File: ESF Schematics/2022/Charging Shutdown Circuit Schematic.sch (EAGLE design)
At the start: 15 parts, among them K1 RELAY_SPST_NO_

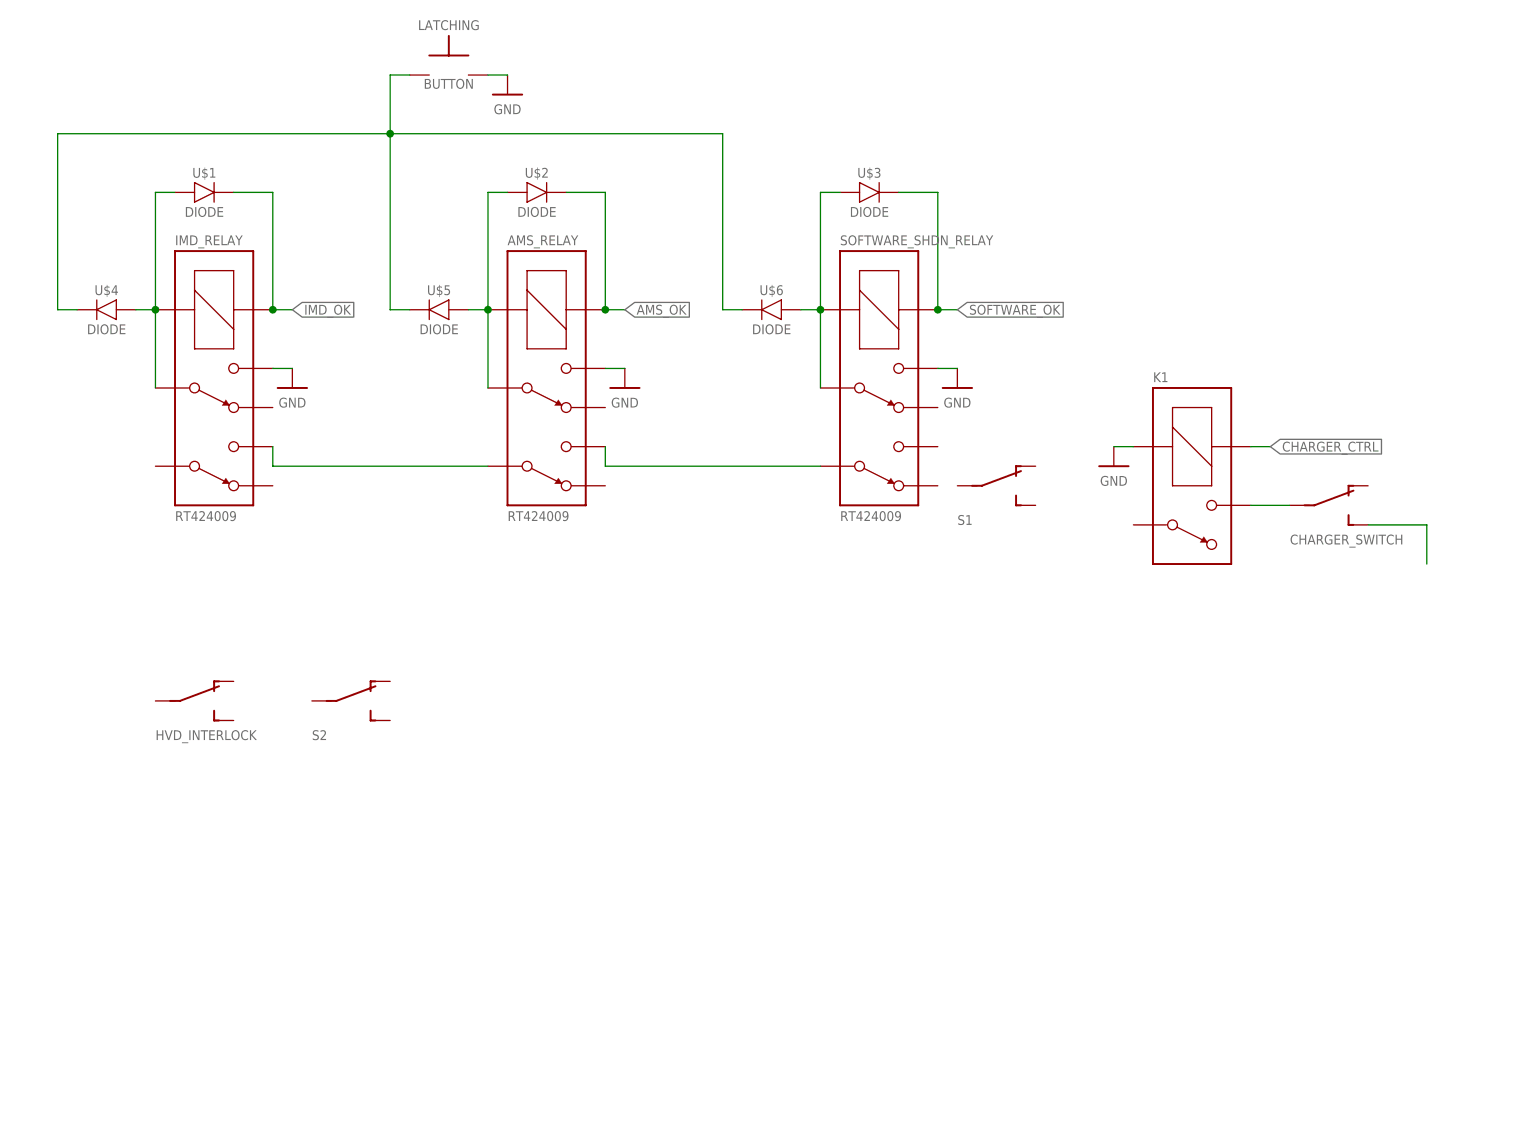
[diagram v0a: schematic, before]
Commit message: Further progress on charging shutdown circuit
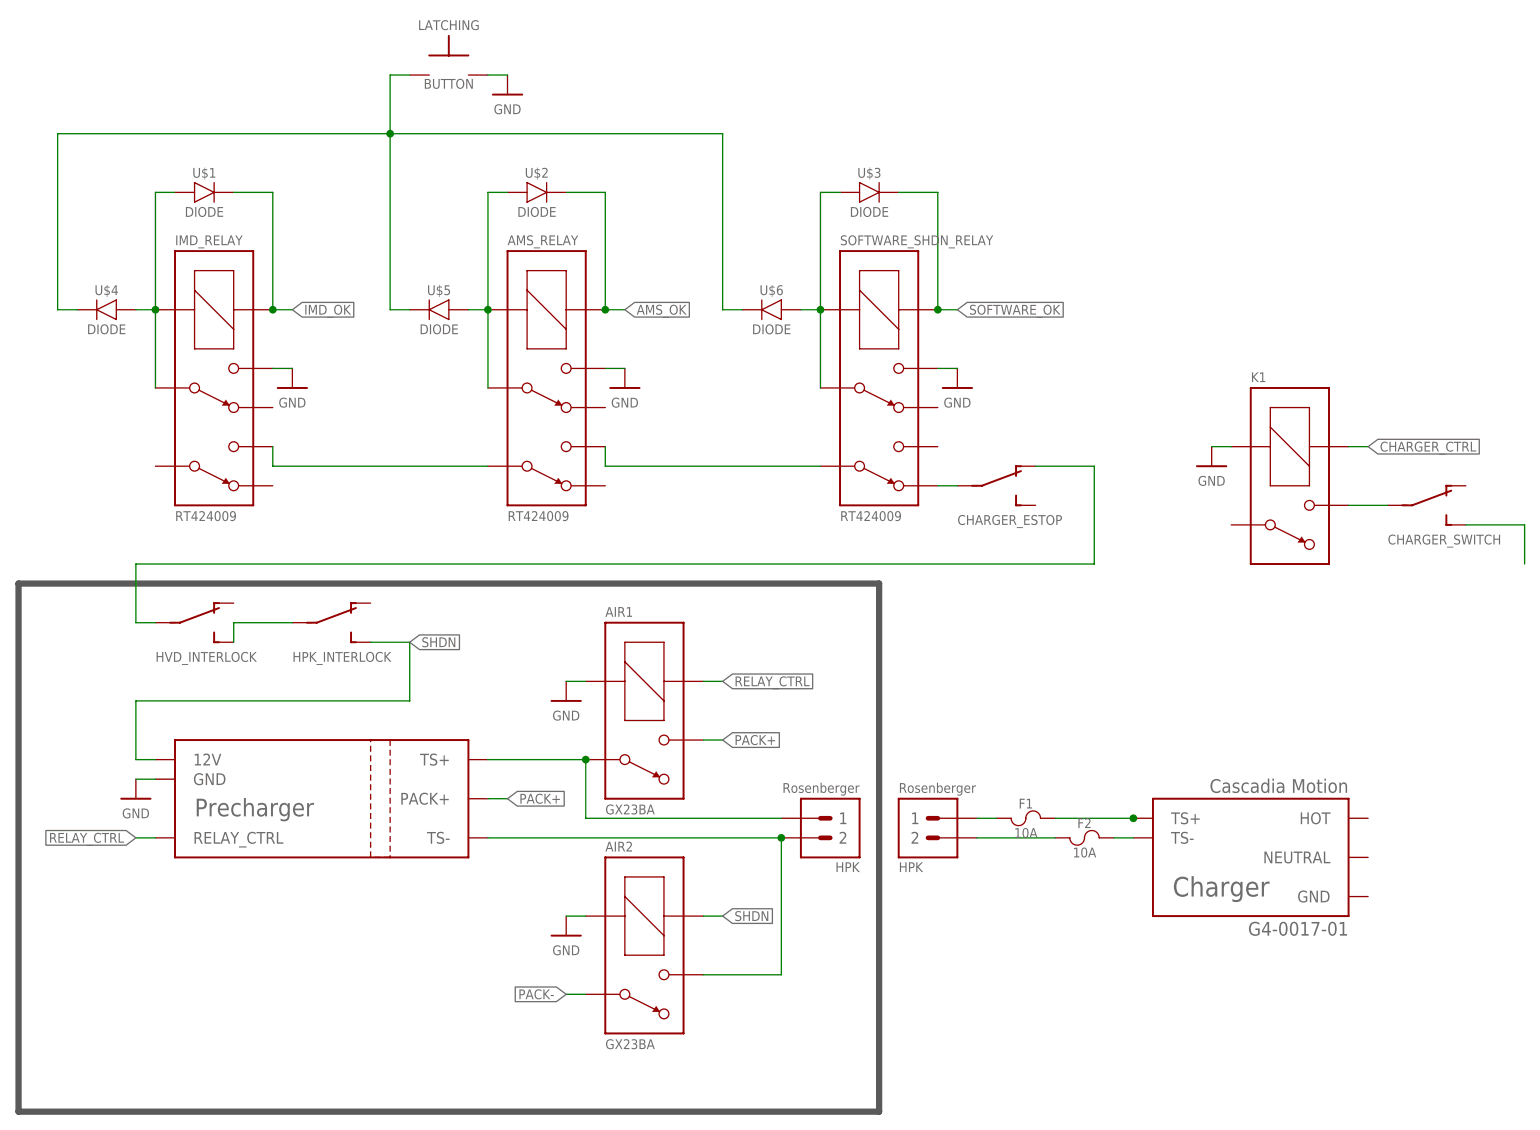
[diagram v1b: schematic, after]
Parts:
- removed S2: SWITCH_SPST, HyTechSymbols:SWITCH_SPST
- added AIR1, AIR2: RELAY_SPST_NO_GX23BA, HyTechSymbolsTemp:RELAY_SPST_NO_GX23BA
- added F1, F2: 10A, HyTechSymbolsTemp:FUSE
- added HPK_INTERLOCK: SWITCH_SPST, HyTechSymbols:SWITCH_SPST
- added J1, J2: CONNECTOR-2_HPK, HyTechSymbolsTemp:CONNECTOR-2_HPK
- added U$7: PRECHARGER, HyTechSymbolsTemp:PRECHARGER
- added U$8: CHARGER_G4-0017-01, HyTechSymbolsTemp:CHARGER_G4-0017-01
- renumbered S1 to CHARGER_ESTOP
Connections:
- new net N$12: AIR1.CONTACT1, J1.1, U$7.TS+
- new net N$13: AIR2.CONTACT2, J1.2, U$7.TS-
- new net N$14: F1.1, J2.1
- new net N$15: F2.1, J2.2
- new net N$16: F1.2, U$8.TS+
- new net N$17: F2.2, U$8.TS-
- new net N$7: CHARGER_ESTOP.P, SOFTWARE_SHDN_RELAY.7
- new net N$8: CHARGER_ESTOP.O, HVD_INTERLOCK.P
- new net N$9: HPK_INTERLOCK.P, HVD_INTERLOCK.S
- new net PACK+: AIR1.CONTACT2, U$7.PACK+
- new net PACK-: AIR2.CONTACT1
- new net RELAY_CTRL: AIR1.COIL-, U$7.RELAY_CTRL
- new net SHDN: AIR2.COIL-, HPK_INTERLOCK.S, U$7.12V
- net GND: now also AIR1.COIL+, AIR2.COIL+, U$7.GND
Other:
- moved on the sheet: CHARGER_SWITCH, HVD_INTERLOCK, K1
